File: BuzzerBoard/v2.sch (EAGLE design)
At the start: 12 parts, among them J1 p0, U1 LM386MX-1/NOPB, U2 Value, U3 LQM2HPN1R5MG0L

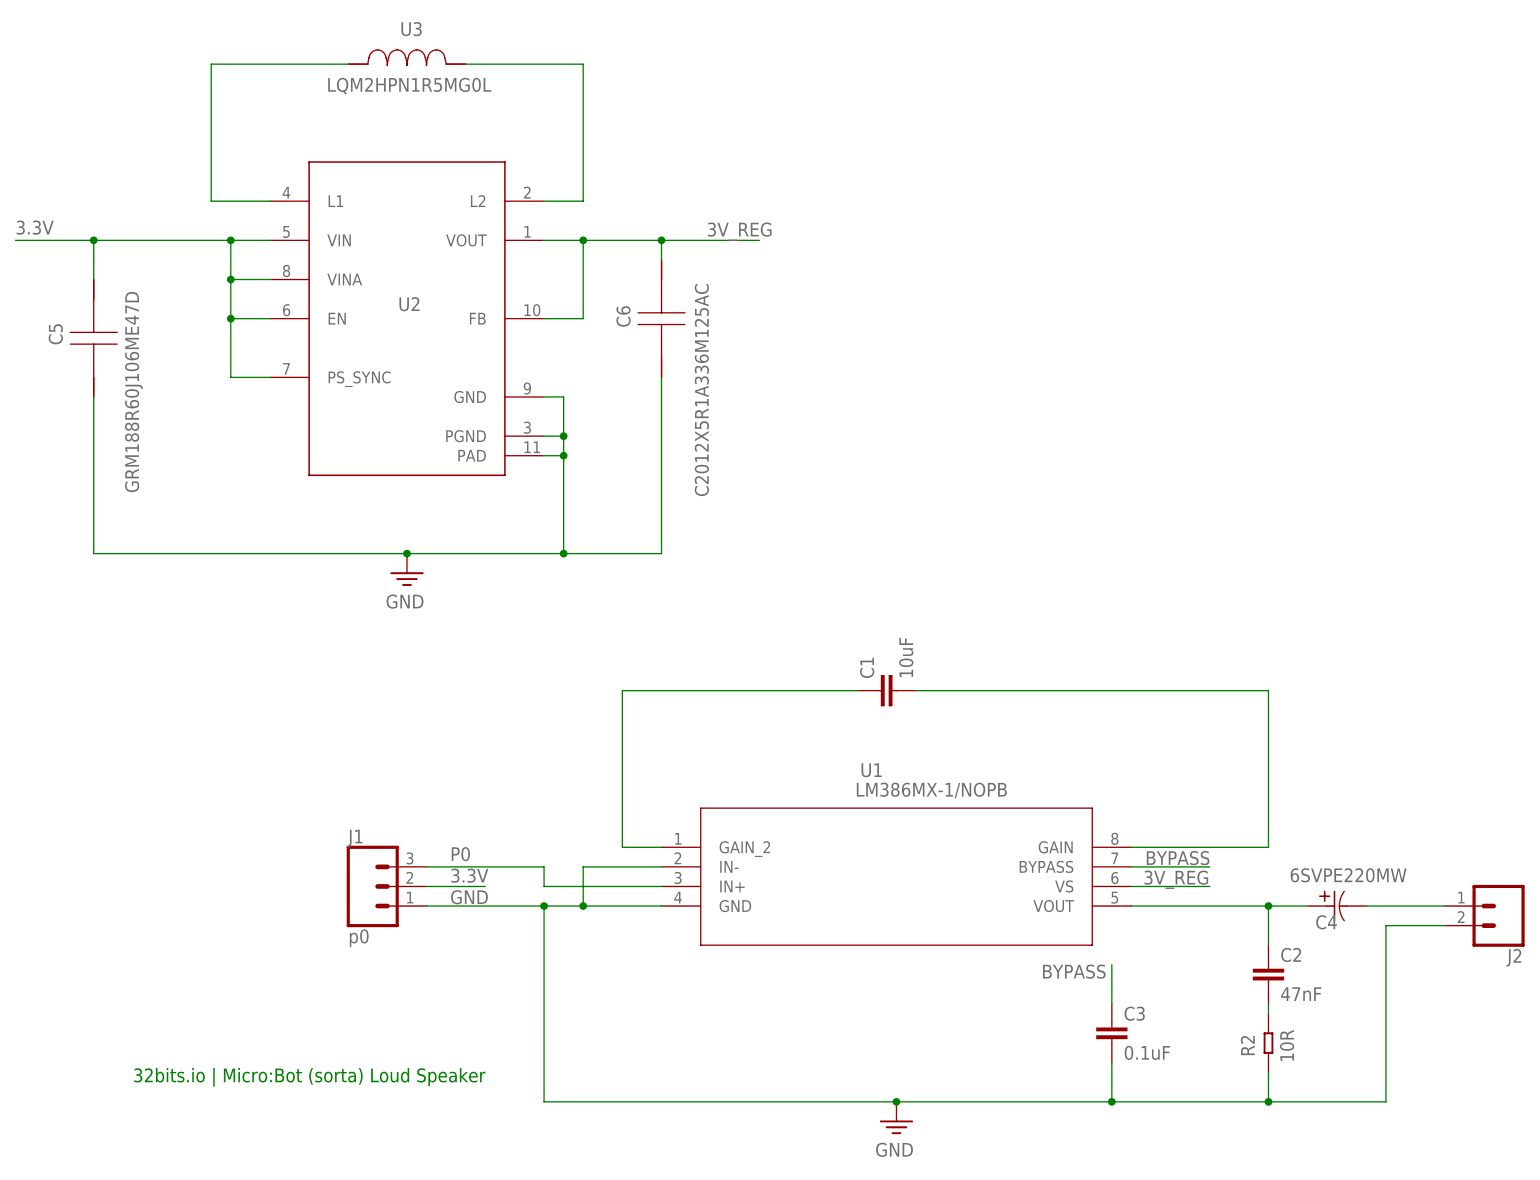
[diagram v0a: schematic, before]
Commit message: progress on the v2 board
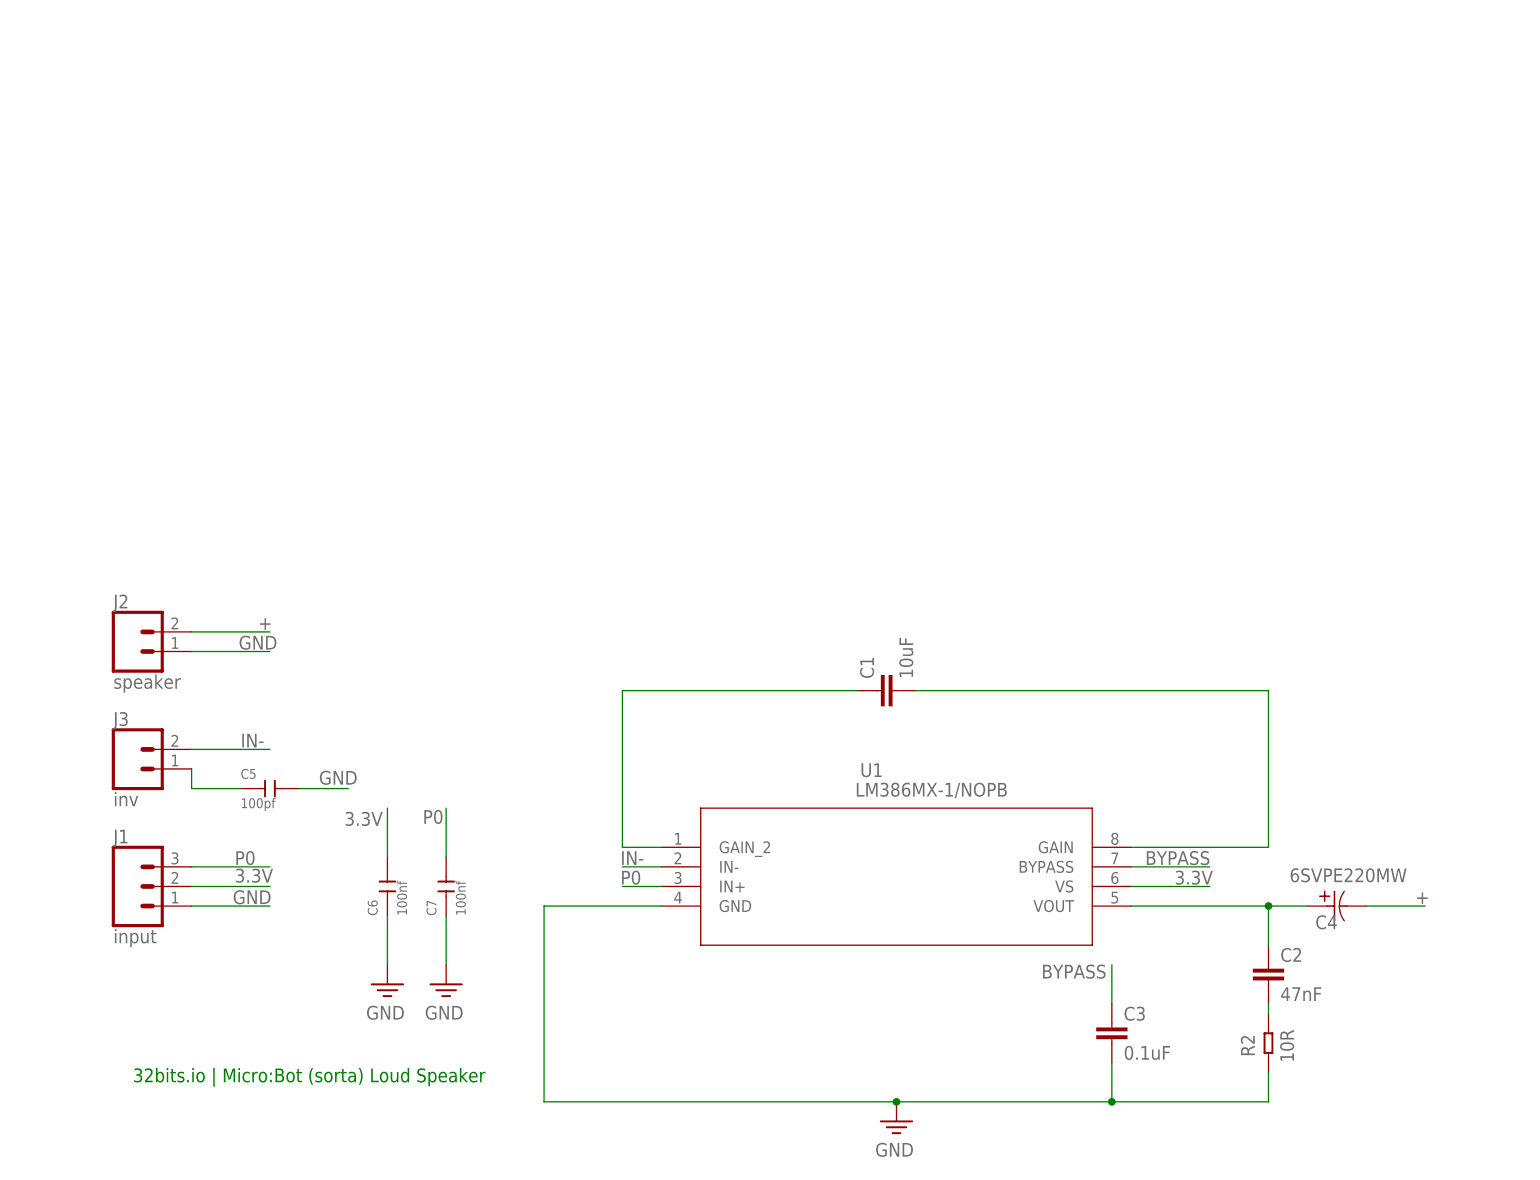
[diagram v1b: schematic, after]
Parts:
- removed U2: Value, BuzzerLib:TPS63001DRCR
- removed U3: LQM2HPN1R5MG0L, BuzzerLib:LQM2HPN1R5MG0L
- added C7: 100nf, Seeed-Capacitor:CERAMIC-100NF-50V-10%-X7R(0603)
- added J3: inv, SparkFun-Connectors:CONN_02
- C5: value GRM188R60J106ME47D -> 100pf; device BuzzerLib:GRM188R60J106ME47D -> Seeed-Capacitor:CERAMIC-100PF-50V-5%-NPO(0603)
- C6: value C2012X5R1A336M125AC -> 100nf; device BuzzerLib:C2012X5R1A336M125AC -> Seeed-Capacitor:CERAMIC-100NF-50V-10%-X7R(0603)
- J1: value p0 -> input
- J2: value (none) -> speaker
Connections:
- removed net 3V_REG: C6.1, U1.VS, U2.FB, U2.VOUT
- removed net N$6: U2.L2, U3.2
- removed net N$7: U2.L1, U3.1
- new net IN-: J3.2, U1.IN-
- new net N$3: C5.1, J3.1
- net +: now also J2.2; no longer J2.1
- net 3.3V: now also C6.2, U1.VS; no longer C5.1, U2.EN, U2.PS_SYNC, U2.VIN, U2.VINA
- net GND: now also C6.1, C7.1, J2.1; no longer C6.2, J2.2, U1.IN-, U2.GND, U2.PAD, U2.PGND
- net P0: now also C7.2
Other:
- moved on the sheet: J1, J2
